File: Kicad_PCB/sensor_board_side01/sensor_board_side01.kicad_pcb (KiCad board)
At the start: 2 copper layers, 30 x 10 mm, 3 parts, among them J1 Conn_01x06_Female, U1 ohmmetr

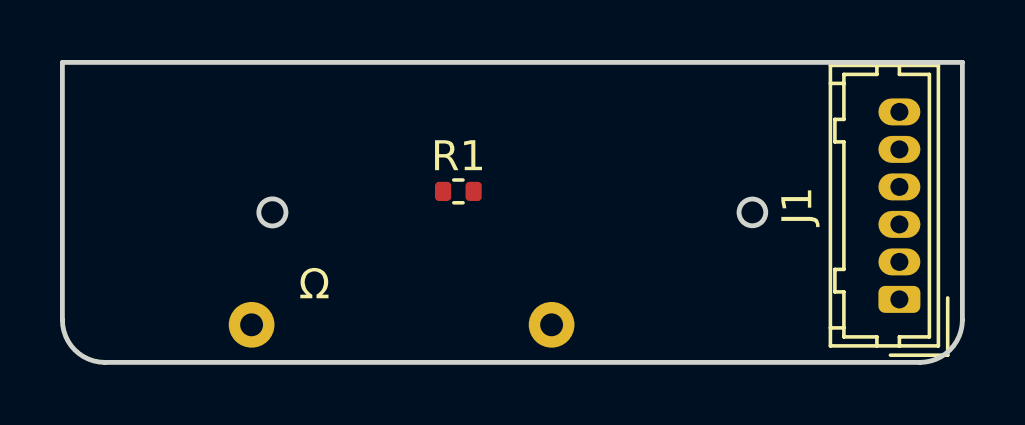
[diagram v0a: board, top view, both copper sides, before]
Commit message: Sensor Board Schematic
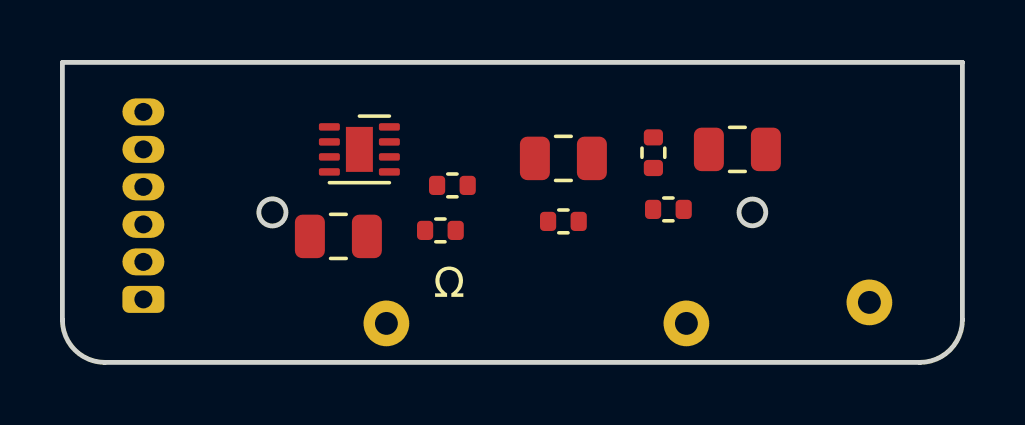
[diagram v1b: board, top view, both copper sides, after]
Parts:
- added C1: 1uF, Capacitor_SMD:C_0805_2012Metric, F.Cu at (164.3, 136.0)
- added C2: 0.1uF, Capacitor_SMD:C_0805_2012Metric, F.Cu at (151.0, 138.9)
- added C3: 10nF, Capacitor_SMD:C_0805_2012Metric, F.Cu at (158.5, 136.3)
- added R2: 1k, Resistor_SMD:R_0402_1005Metric, F.Cu at (158.5, 138.4)
- added R3: 100k, Resistor_SMD:R_0402_1005Metric, F.Cu at (154.8, 137.2)
- added R4: 1M, Resistor_SMD:R_0402_1005Metric, F.Cu at (161.5, 136.1)
- added R5: 10k, Resistor_SMD:R_0402_1005Metric, F.Cu at (154.4, 138.7)
- added U2: AT42QT1012-M, Package_DFN_QFN:DFN-8-1EP_2x2mm_P0.5mm_EP0.9x1.5mm, F.Cu at (151.7, 136.0)
- added U3: sensor, cup_toch:toch_sens, F.Cu at (168.7, 141.1)
- J1: moved to B.Cu
- moved J1 25.2 mm to (144.5, 141.0)
- moved R1 7.03 mm to (162.0, 138.0)
- moved U1 4.49 mm to (152.6, 141.8)
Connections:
- J1 pad 3: unconnected-(J1-Pad3) -> Net-(J1-Pad3)
